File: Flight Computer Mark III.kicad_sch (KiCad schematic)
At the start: 69 parts, among them J1 Conn_01x02, J2 USB_C_Receptacle_USB2.0_16P, Q1 PSMN075-100MSE, Q2 PSMN075-100MSE, Q3 PSMN075-100MSE, U1 CP2102N-Axx-xQFN20

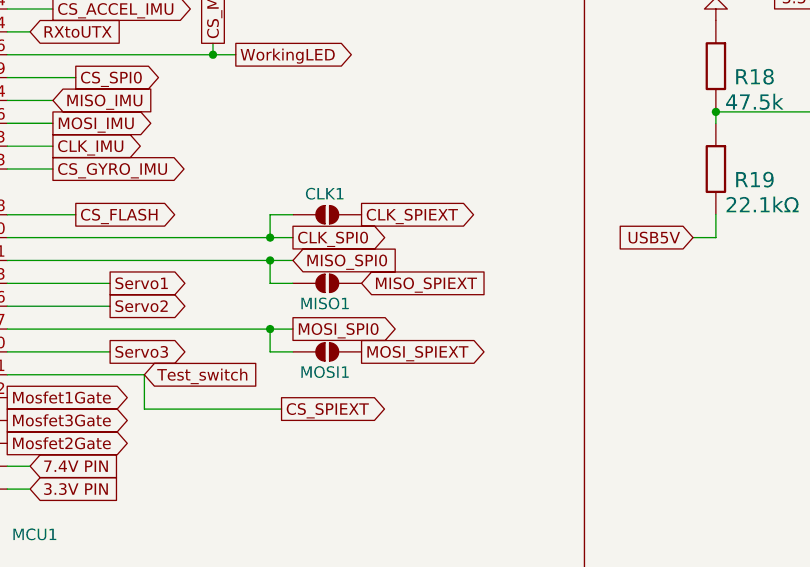
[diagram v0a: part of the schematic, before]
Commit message: lol
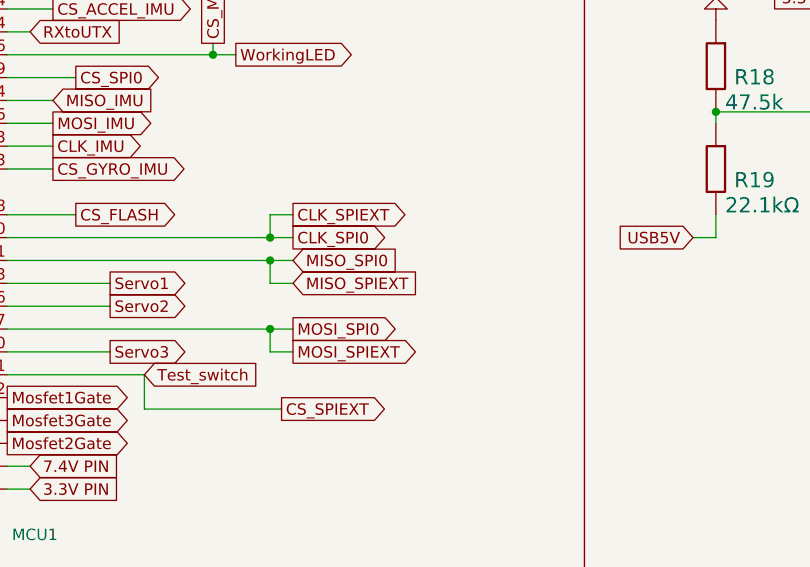
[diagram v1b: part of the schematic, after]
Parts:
- removed CLK1, MISO1, MOSI1: SolderJumper_2_Open, Capacitor_SMD:C_0603_1608Metric, symbol Jumper:SolderJumper_2_Open
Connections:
- net CLK_SPIEXT is gone; now on net CLK_SPI0: SPI_EXT1.6 (Pin_6)
- net MISO_SPIEXT is gone; now on net MISO_SPI0: SPI_EXT1.4 (Pin_4)
- net MOSI_SPIEXT is gone; now on net MOSI_SPI0: SPI_EXT1.3 (Pin_3)
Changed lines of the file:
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@@
 	(global_label "CLK_SPIEXT"
 		(shape output)
-		(at 273.05 60.96 0)
+		(at 265.43 60.96 0)
 		(effects
 			(font
@@
 		)
 		(property "Intersheetrefs" "${INTERSHEET_REFS}"
-			(at 273.05 60.96 0)
+			(at 265.43 60.96 0)
 			(effects
 				(font
@@
 	(global_label "MOSI_SPIEXT"
 		(shape output)
-		(at 273.05 76.2 0)
+		(at 265.43 76.2 0)
 		(effects
 			(font
@@
 		)
 		(property "Intersheetrefs" "${INTERSHEET_REFS}"
-			(at 273.05 76.2 0)
+			(at 265.43 76.2 0)
 			(effects
 				(font
@@
 	(global_label "MISO_SPIEXT"
 		(shape input)
-		(at 273.05 68.58 0)
+		(at 265.43 68.58 0)
 		(effects
 			(font
@@
 		)
 		(property "Intersheetrefs" "${INTERSHEET_REFS}"
-			(at 273.05 68.58 0)
+			(at 265.43 68.58 0)
 			(effects
 				(font
@@
 	)
 	(symbol
-		(lib_id "Jumper:SolderJumper_2_Open")
-		(at 269.24 60.96 0)
-		(unit 1)
-		(exclude_from_sim yes)
-		(in_bom no)
-		(on_board yes)
-		(dnp no)
-		(property "Reference" "CLK1"
-			(at 268.986 58.674 0)
-			(effects
-				(font
-					(size 1.27 1.27)
-				)
-			)
-		)
-		(property "Value" "SolderJumper_2_Open"
-			(at 268.986 58.42 0)
-			(effects
-				(font
-					(size 1.27 1.27)
-				)
-				(hide yes)
-			)
-		)
-		(property "Footprint" "Capacitor_SMD:C_0603_1608Metric"
-			(at 269.24 60.96 0)
-			(effects
-				(font
-					(size 1.27 1.27)
-				)
-				(hide yes)
-			)
-		)
-		(property "Datasheet" "~"
-			(at 269.24 60.96 0)
-			(effects
-				(font
-					(size 1.27 1.27)
-				)
-				(hide yes)
-			)
-		)
-		(property "Description" "Solder Jumper, 2-pole, open"
-			(at 269.24 60.96 0)
-			(effects
-				(font
-					(size 1.27 1.27)
-				)
-				(hide yes)
-			)
-		)
-		(pin "2"
-		)
-		(pin "1"
-		)
-		(instances
-			(project "Flight Computer Mark III"
-				(path "/0bad6c6f-d77b-4b1f-bd5d-3c971ec5e274"
-					(reference "CLK1")
-					(unit 1)
-				)
-			)
-		)
-	)
-	(symbol
 		(lib_id "Flight Computer:Pyro-Pad")
 		(at 167.64 193.04 90)
@@
 	)
 	(symbol
-		(lib_id "Jumper:SolderJumper_2_Open")
-		(at 269.24 76.2 0)
-		(unit 1)
-		(exclude_from_sim yes)
-		(in_bom no)
-		(on_board yes)
-		(dnp no)
-		(property "Reference" "MOSI1"
-			(at 268.986 78.486 0)
-			(effects
-				(font
-					(size 1.27 1.27)
-				)
-			)
-		)
-		(property "Value" "SolderJumper_2_Open"
-			(at 268.986 73.66 0)
-			(effects
-				(font
-					(size 1.27 1.27)
-				)
-				(hide yes)
-			)
-		)
-		(property "Footprint" "Capacitor_SMD:C_0603_1608Metric"
-			(at 269.24 76.2 0)
-			(effects
-				(font
-					(size 1.27 1.27)
-				)
-				(hide yes)
-			)
-		)
-		(property "Datasheet" "~"
-			(at 269.24 76.2 0)
-			(effects
-				(font
-					(size 1.27 1.27)
-				)
-				(hide yes)
-			)
-		)
-		(property "Description" "Solder Jumper, 2-pole, open"
-			(at 269.24 76.2 0)
-			(effects
-				(font
-					(size 1.27 1.27)
-				)
-				(hide yes)
-			)
-		)
-		(pin "2"
-		)
-		(pin "1"
-		)
-		(instances
-			(project ""
-				(path "/0bad6c6f-d77b-4b1f-bd5d-3c971ec5e274"
-					(reference "MOSI1")
-					(unit 1)
-				)
-			)
-		)
-	)
-	(symbol
 		(lib_name "CGA0402X5R226M100GT_1_1")
 		(lib_id "CGA0402X5R226M100GT_1")
@@
 					(unit 1)
 				)
-			)
-		)
-	)
-	(symbol
-		(lib_id "Jumper:SolderJumper_2_Open")
-		(at 269.24 68.58 0)
-		(unit 1)
-		(exclude_from_sim yes)
-		(in_bom no)
-		(on_board yes)
-		(dnp no)
-		(property "Reference" "MISO1"
-			(at 268.986 70.866 0)
-			(effects
-				(font
-					(size 1.27 1.27)
-				)
-			)
-		)
-		(property "Value" "SolderJumper_2_Open"
-			(at 268.986 66.04 0)
-			(effects
-				(font
-					(size 1.27 1.27)
-				)
-				(hide yes)
-			)
-		)
-		(property "Footprint" "Capacitor_SMD:C_0603_1608Metric"
-			(at 269.24 68.58 0)
-			(effects
-				(font
-					(size 1.27 1.27)
-				)
-				(hide yes)
-			)
-		)
-		(property "Datasheet" "~"
-			(at 269.24 68.58 0)
-			(effects
-				(font
-					(size 1.27 1.27)
-				)
-				(hide yes)
-			)
-		)
-		(property "Description" "Solder Jumper, 2-pole, open"
-			(at 269.24 68.58 0)
-			(effects
-				(font
-					(size 1.27 1.27)
-				)
-				(hide yes)
-			)
-		)
-		(pin "2"
-		)
-		(pin "1"
-		)
-		(instances
-			(project "Flight Computer Mark III"
-				(path "/0bad6c6f-d77b-4b1f-bd5d-3c971ec5e274"
-					(reference "MISO1")
-					(unit 1)
-				)
